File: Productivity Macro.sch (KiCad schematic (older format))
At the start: 34 parts, among them SW1 SW_Push, SW2 Rotary_Encoder_Switch, SW3 Rotary_Encoder_Switch, U1 ATmega32U4-AU, Y1 16Mhz

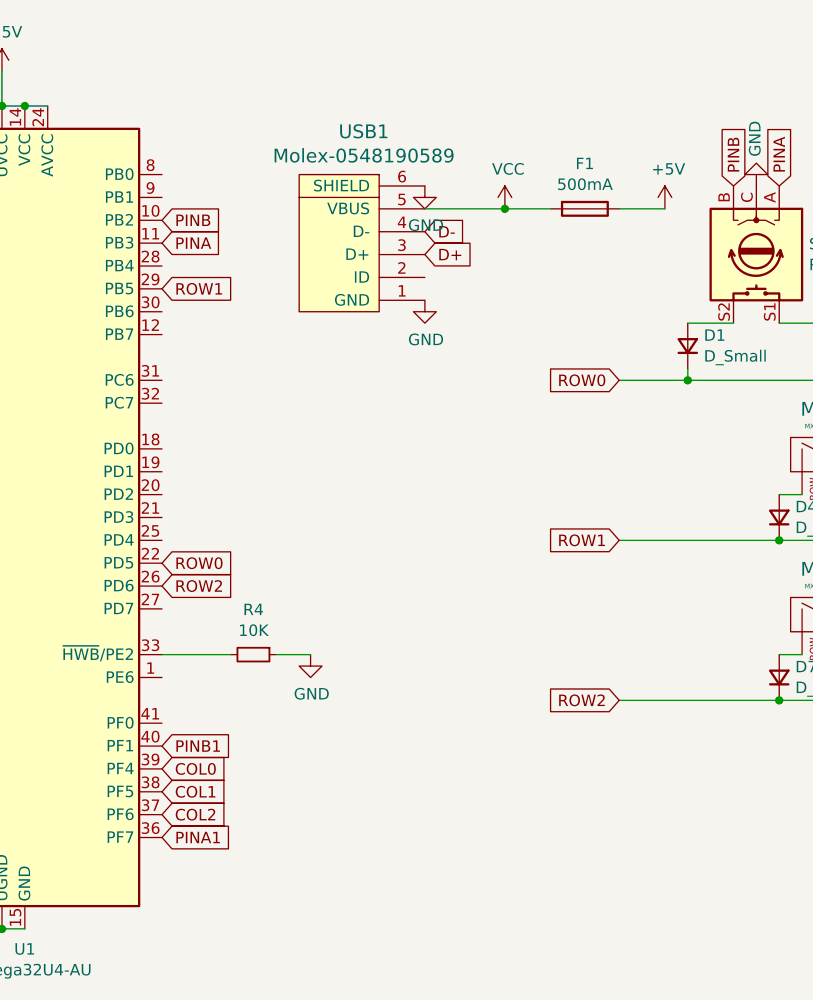
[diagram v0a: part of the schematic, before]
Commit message: The beginning of the trackball
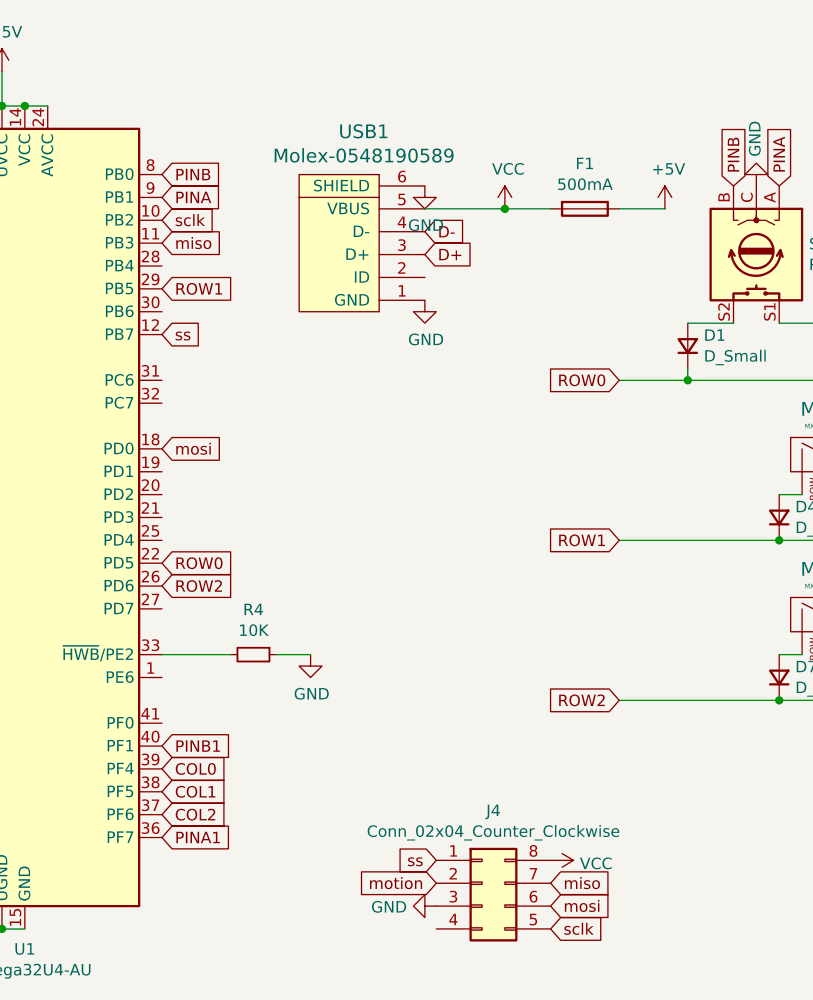
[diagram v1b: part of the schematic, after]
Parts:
- added J4: Conn_02x04_Counter_Clockwise, Connector_PinSocket_2.00mm:PinSocket_2x04_P2.00mm_Vertical, symbol Connector_Generic:Conn_02x04_Counter_Clockwise
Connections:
- net GND: now also J4.3 (Pin_3)
- net PINA: now also U1.9 (PB1); no longer U1.11 (PB3)
- net PINB: now also U1.8 (PB0); no longer U1.10 (PB2)
- net VCC: now also J4.8 (Pin_8)
- net ss: now reaches U1.12 (PB7)
- net ss: now also J4.1 (Pin_1)
- net mosi: now reaches U1.18 (PD0)
- net mosi: now also J4.6 (Pin_6)
- new net miso: J4.7 (Pin_7), U1.11 (PB3)
- new net motion: J4.2 (Pin_2)
- new net sclk: J4.5 (Pin_5), U1.10 (PB2)
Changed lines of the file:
@@
 Text GLabel 4900 3200 2    50   Input ~ 0
 ROW2
-Text GLabel 4900 1700 2    50   Input ~ 0
+Text GLabel 4900 1500 2    50   Input ~ 0
 PINA
-Text GLabel 4900 1600 2    50   Input ~ 0
+Text GLabel 4900 1400 2    50   Input ~ 0
 PINB
 Text GLabel 7600 1450 1    50   Input ~ 0
@@
 	1    0    0    -1
 $EndComp
+$Comp
+L Connector_Generic:Conn_02x04_Counter_Clockwise J4
+U 1 1 60BB48DB
+P 6300 4500
+F 0 "J4" H 6350 4817 50  0000 C CNN
+F 1 "Conn_02x04_Counter_Clockwise" H 6350 4726 50  0000 C CNN
+F 2 "Connector_PinSocket_2.00mm:PinSocket_2x04_P2.00mm_Vertical" H 6300 4500 50  0001 C CNN
+F 3 "~" H 6300 4500 50  0001 C CNN
+	1    6300 4500
+	1    0    0    -1
+$EndComp
+Text GLabel 6100 4400 0    50   Input ~ 0
+ss
+Text GLabel 6100 4500 0    50   Input ~ 0
+motion
+Text GLabel 6600 4500 2    50   Input ~ 0
+miso
+Text GLabel 6600 4600 2    50   Input ~ 0
+mosi
+Text GLabel 6600 4700 2    50   Input ~ 0
+sclk
+$Comp
+L power:GND #PWR0117
+U 1 1 60BB7D4F
+P 6100 4600
+F 0 "#PWR0117" H 6100 4350 50  0001 C CNN
+F 1 "GND" V 6105 4472 50  0000 R CNN
+F 2 "" H 6100 4600 50  0001 C CNN
+F 3 "" H 6100 4600 50  0001 C CNN
+	1    6100 4600
+	0    1    1    0
+$EndComp
+$Comp
+L power:VCC #PWR0118
+U 1 1 60BB8B38
+P 6600 4400
+F 0 "#PWR0118" H 6600 4250 50  0001 C CNN
+F 1 "VCC" V 6615 4528 50  0000 L CNN
+F 2 "" H 6600 4400 50  0001 C CNN
+F 3 "" H 6600 4400 50  0001 C CNN
+	1    6600 4400
+	0    1    1    0
+$EndComp
+Text GLabel 4900 1600 2    50   Input ~ 0
+sclk
+Text GLabel 4900 1700 2    50   Input ~ 0
+miso
+Text GLabel 4900 2600 2    50   Input ~ 0
+mosi
+Text GLabel 4900 2100 2    50   Input ~ 0
+ss
 $EndSCHEMATC
